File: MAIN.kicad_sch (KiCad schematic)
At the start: 3 parts

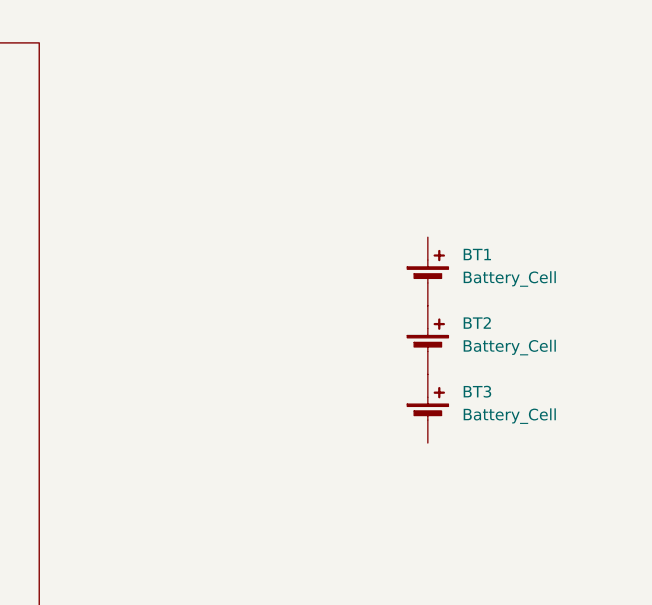
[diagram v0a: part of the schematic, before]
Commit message: REV1 PCB that was sent to production (PCBWAY)
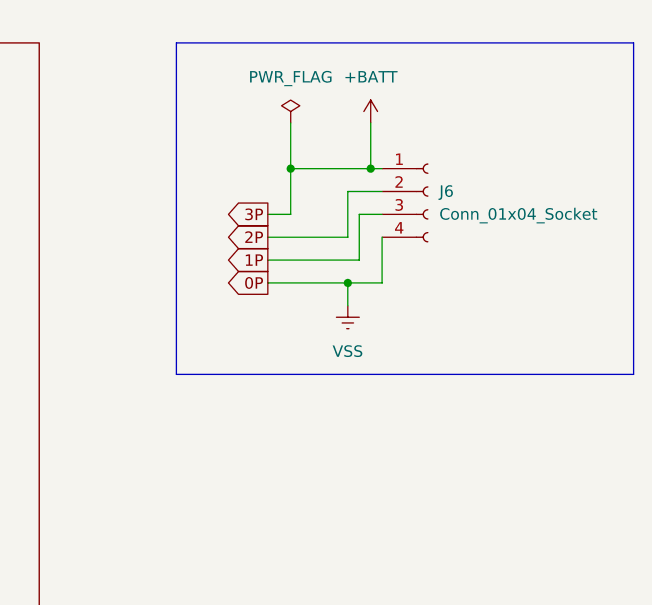
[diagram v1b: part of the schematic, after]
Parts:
- removed BT1, BT2, BT3: Battery_Cell, symbol Device:Battery_Cell
- added J6: Conn_01x04_Socket, Connector_JST:JST_XH_B4B-XH-A_1x04_P2.50mm_Vertical, symbol Connector:Conn_01x04_Socket
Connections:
- new net +BATT: J6.1 (Pin_1)
- new net 1P: J6.3 (Pin_3)
- new net 2P: J6.2 (Pin_2)
- new net VSS: J6.4 (Pin_4)
